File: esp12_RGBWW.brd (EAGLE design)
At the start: 49.5 x 50.5 mm, 29 parts

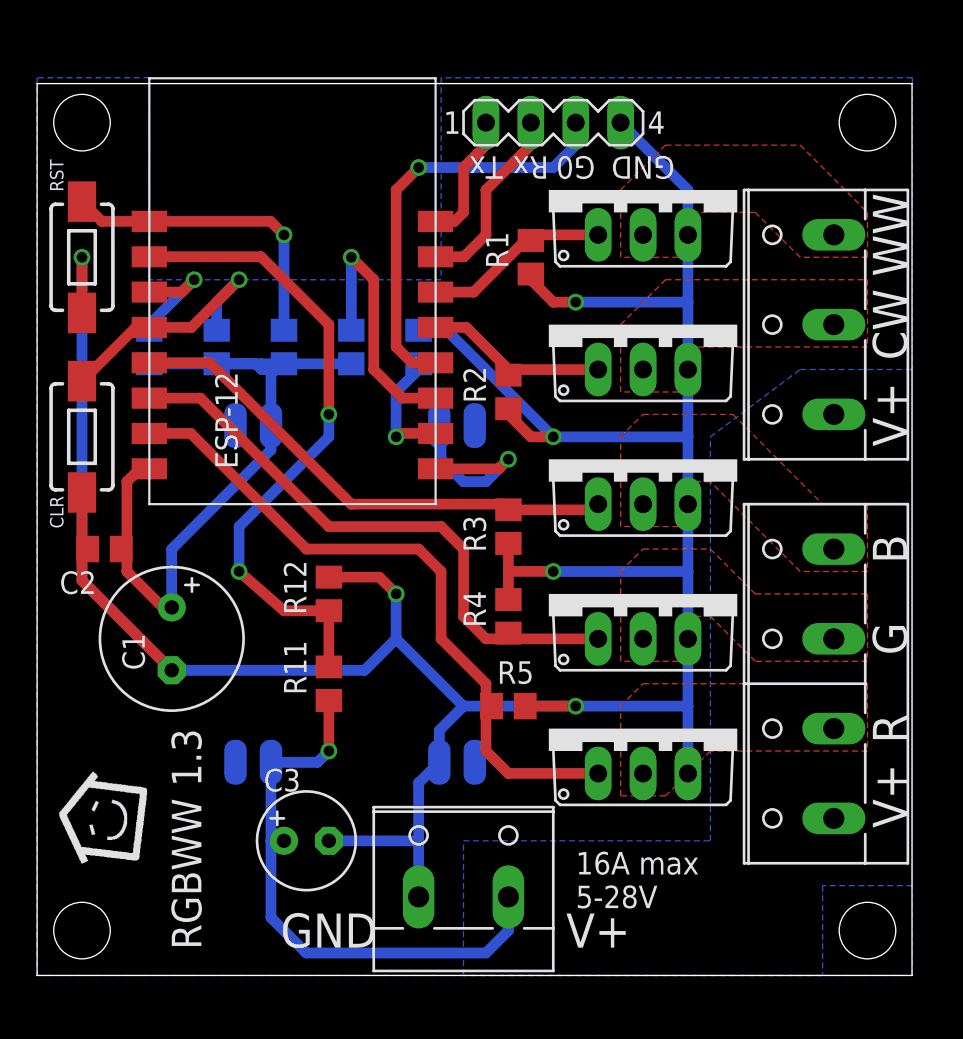
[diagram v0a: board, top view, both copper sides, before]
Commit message: updated schematics and board v1.5
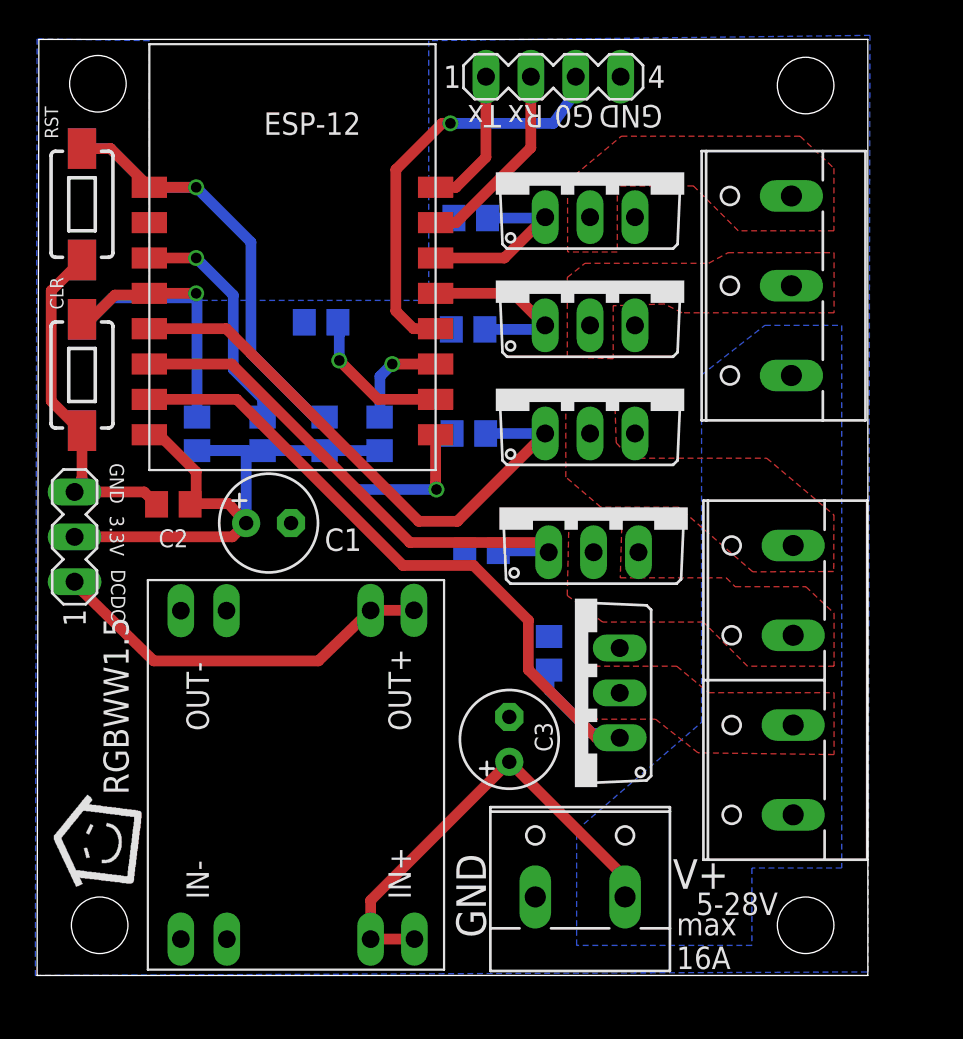
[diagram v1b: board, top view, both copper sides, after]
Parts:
- removed DC_CONVERTER: CN1594THROUGH-HOLE, CN1594_smd:CN1594
- removed R11: 10k, rcl:R0805
- removed R12: 1k, rcl:R0805
- added CLR1, RST1: (no value), SparkFun-Electromechanical:TACTILE-SWITCH-1101NE
- added SV1: (no value), con-lstb:MA03-1
- added U$2: XM1584, XM1584:XM1584-TH
- C1: device rcl:E3,5-8 -> resistor:E2,5-6
- moved C3 12.8 mm to (26.7, 13.4), turned to 90 degrees
- moved C1 8.54 mm to (13.1, 25.6), turned to 0 degrees
- moved R9 8.07 mm to (12.8, 30.6)
- moved VCC 6.60 mm to (30.7, 5.08)
- moved R3 5.73 mm to (24.4, 30.7), flipped to the bottom, turned to 0 degrees
- moved R6 5.70 mm to (16.1, 37.0), turned to 0 degrees
- moved IRLZ44N-G 5.64 mm to (31.5, 26.5)
- moved R10 5.42 mm to (16.3, 30.6)
- moved R7 5.16 mm to (19.4, 30.6)
- moved R8 5.03 mm to (9.05, 30.6)
- moved IRLZ44N-B 5.00 mm to (31.3, 33.2)
- moved C2 4.65 mm to (7.71, 26.7)
- moved IRLZ44N-R 4.36 mm to (30.4, 16.0), turned to 90 degrees
- moved R2 4.21 mm to (24.4, 36.6), flipped to the bottom, turned to 0 degrees
- moved R1 4.06 mm to (24.5, 42.9), flipped to the bottom, turned to 180 degrees
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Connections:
- removed net N$21: ESP-12.10, R11.1, R12.2
- new net DCDC+: SV1.1, U$2.OUT+(1), U$2.OUT+(2)
- net +12V: now also U$2.IN+(1), U$2.IN+(2); no longer DC_CONVERTER.IN+(1), R11.2
- net +3V3: now also SV1.2; no longer DC_CONVERTER.OUT+(1)
- net GND: now also CLR1.1, RST1.1, SV1.3, U$2.IN-(1), U$2.IN-(2), U$2.OUT-(1), U$2.OUT-(2); no longer DC_CONVERTER.IN-(2), DC_CONVERTER.OUT-(2), R12.1
- net N$1: now also CLR1.2
- net N$12: now also RST1.2
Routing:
- net GND: track 192.9 -> 27.2 mm, vias 7 -> 1
- net N$21: track 36.9 -> 0.00 mm, vias 2 -> 0
- net DCDC+: track 0.00 -> 22.2 mm
- net N$12: track 17.6 -> 31.1 mm
- net N$3: track 15.2 -> 5.75 mm
- net +3V3: track 43.5 -> 36.2 mm
- net N$1: track 14.7 -> 21.2 mm
- net +12V: track 32.6 -> 26.1 mm, vias 1 -> 0
- net N$2: track 6.74 -> 13.2 mm
- net RGB-G: track 33.7 -> 29.9 mm
- net RGB-R: track 38.7 -> 42.5 mm
- net RGB-B: track 29.6 -> 32.3 mm
- net N$7: track 6.96 -> 8.53 mm
- net RGB-WW: track 11.4 -> 10.4 mm
- net N$8: track 7.40 -> 8.11 mm
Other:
- board size 49.5 x 50.5 mm -> 47 x 53 mm
- board text added: "3.3V"
- board text added: "DCDC"
- board text added: "RGBWW1.5"
- board text added: "max 16A"
- board text removed: "16A max"
- board text removed: "RGBWW 1.3"
